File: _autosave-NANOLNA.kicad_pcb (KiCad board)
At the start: 4 copper layers, 25 x 15 mm, 11 parts, among them J1 USB_C_Receptacle_PowerOnly_6P, J2 Conn_Coaxial, J4 Conn_Coaxial, U1 PMA3-83LN_

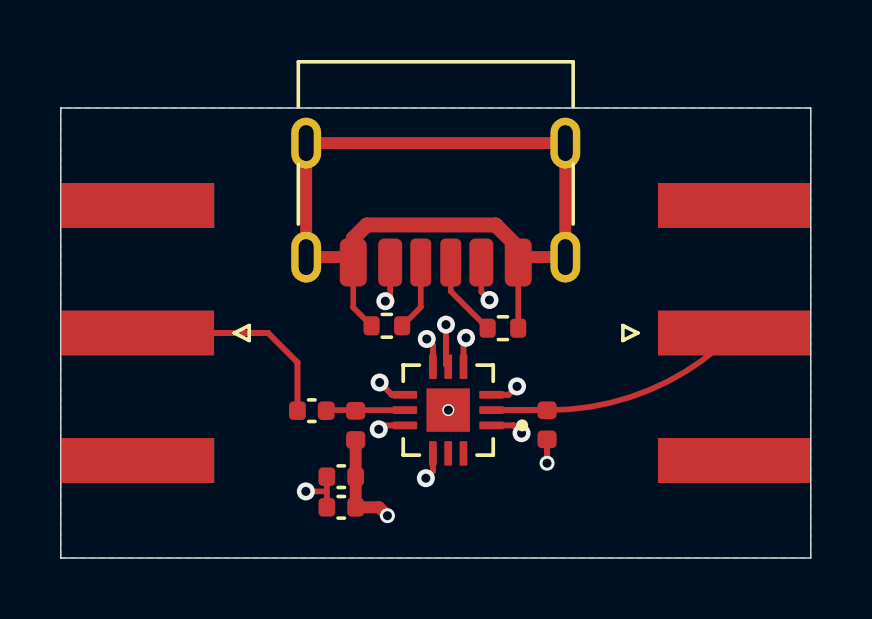
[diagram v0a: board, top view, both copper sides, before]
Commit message: made it nano-er
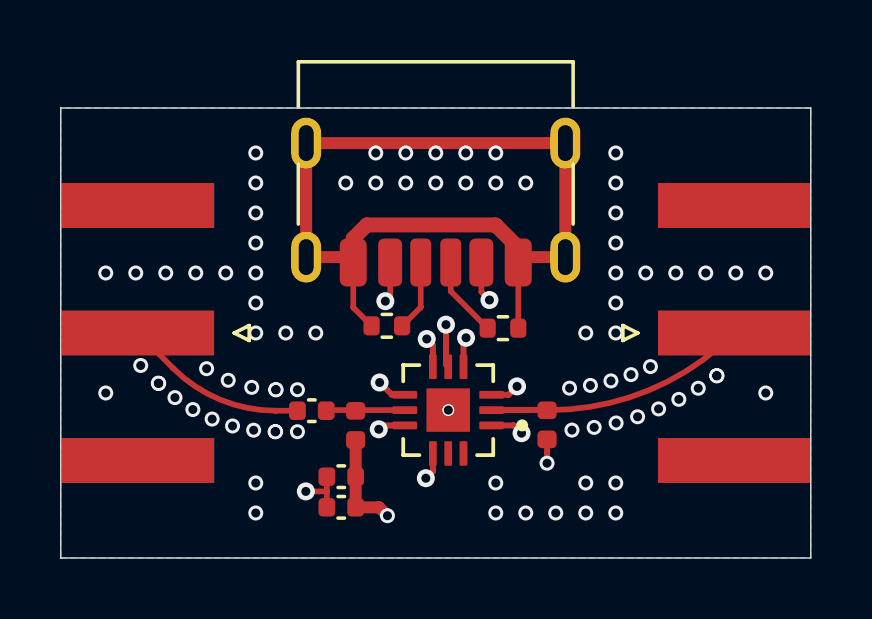
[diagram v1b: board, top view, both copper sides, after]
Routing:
- net /RF OUT: track 7.33 -> 6.16 mm
- net GND: vias 3 -> 85
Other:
- board text added: "{ "ViaStitching": "0.2", "stitch_zone_0": { "HSpacing": "0.7", "VSpacing": "0.6", "HOffset": "0", "VOffset": "0", "Clearance": "0.7", "Randomize": false } }"
- board text added: "{ "ViaStitching": "0.2", "stitch_zone_0": { "HSpacing": "1", "VSpacing": "1", "HOffset": "0", "VOffset": "0", "Clearance": "00.5", "Randomize": false } }"
